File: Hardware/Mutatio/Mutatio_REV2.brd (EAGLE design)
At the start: 47.2 x 50 mm, 39 parts, among them IC1 DS3231/SO, IC2 74AUC1G14DBV, J1 MICRO-SDCARD-CONNECTOR-330006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

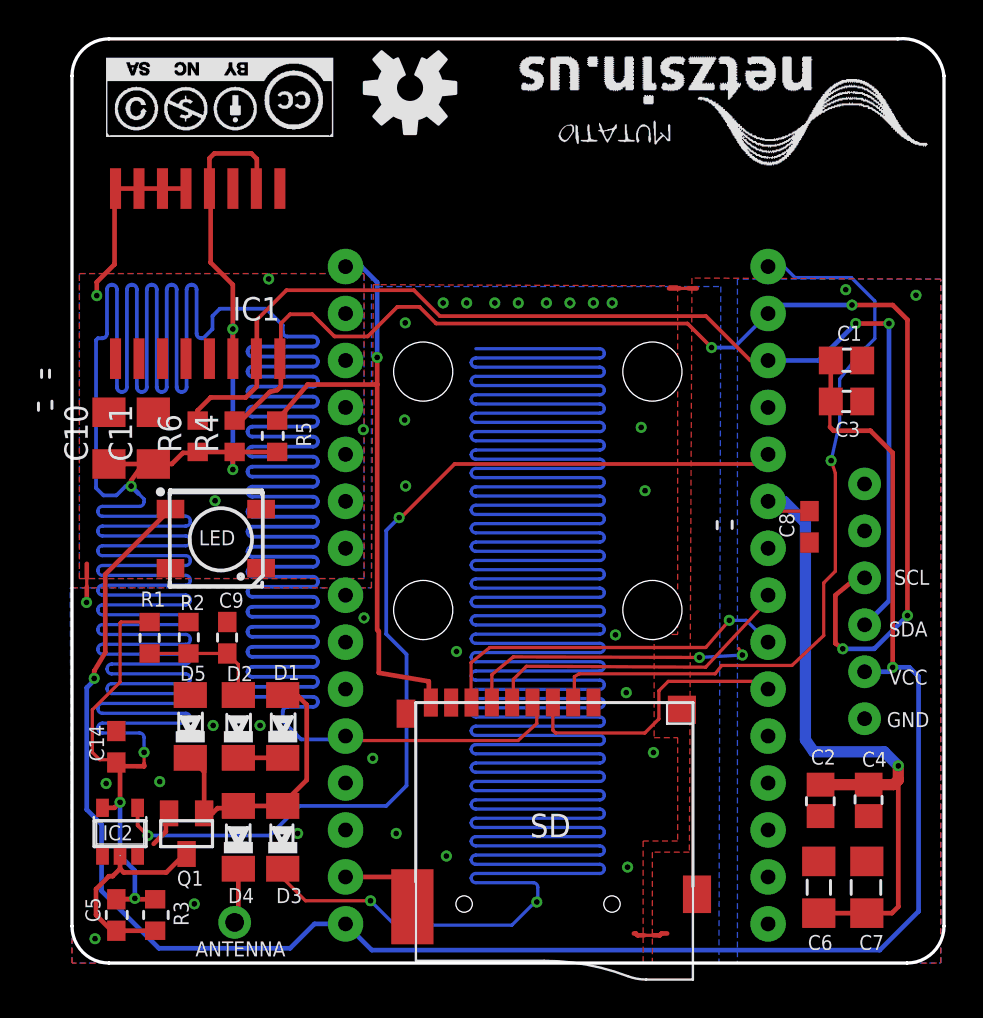
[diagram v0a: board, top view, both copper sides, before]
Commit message: finished revision 2
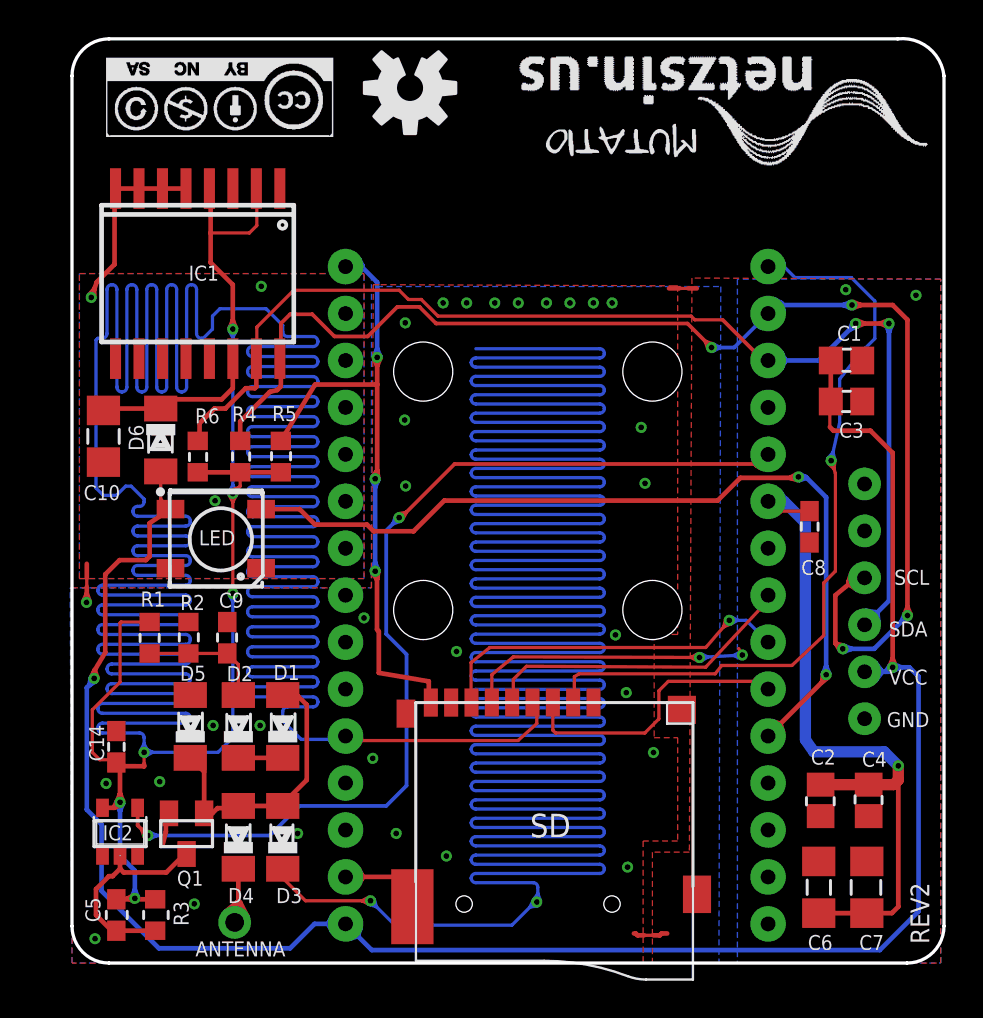
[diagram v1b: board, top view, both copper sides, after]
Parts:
- removed C11: 100uF, resistor:C1206
- added D6: (no value), diode:MINIMELF
- moved R4 1.14 mm to (9.10, 27.4)
- moved R5 1.12 mm to (11.3, 27.4)
- moved R6 1.10 mm to (6.80, 27.4)
- moved C10 0.32 mm to (1.70, 28.5), turned to 270 degrees
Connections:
- new net N$6: C10.1, D6.C, IC1.14
- net +3V3: no longer C10.1, C11.1, IC1.14
- net +5V: now also D6.A
- net GND: no longer C11.2
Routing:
- net WS2812_DATA: track 0.00 -> 53.9 mm, vias 0 -> 2
- net SCL: track 69.5 -> 86.3 mm
- net +5V: track 105.4 -> 121.2 mm
- net +3V3: track 439.6 -> 454.1 mm
- net SDA: track 62.0 -> 73.6 mm
- net !SDCARD_DETECT: track 33.5 -> 43.5 mm, vias 1 -> 3
- net N$6: track 0.00 -> 9.27 mm
- net GND: track 31.8 -> 39.0 mm
- net SIGNAL: track 53.5 -> 60.4 mm
- net VDD: track 24.1 -> 30.2 mm
- net BOARDANTENNA: track 449.8 -> 454.7 mm
- net SPI_MISO: track 19.7 -> 24.0 mm
- net SD_CSN: track 41.7 -> 46.0 mm
- net N$3: track 2.98 -> 5.84 mm
- net SPI_MOSI: track 15.4 -> 17.3 mm
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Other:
- board text added: "22. MAR. 2016"
- board text added: "REV2"
- board text added: "REVISION 2"
- board text removed: "17. JAN. 2016"
- board text removed: "REVISION 1"
